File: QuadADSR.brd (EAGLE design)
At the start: 66.6 x 100 mm, 75 parts, among them IC1 74AC32D, IC5 MCP6004D, Q1 20MHz, T1 2N3904, T2 2N3904, T3 2N3904, T4 2N3904, U1 ATMEGA328P, U2 DUAL_OPAMP, U3 7805, U4 4051

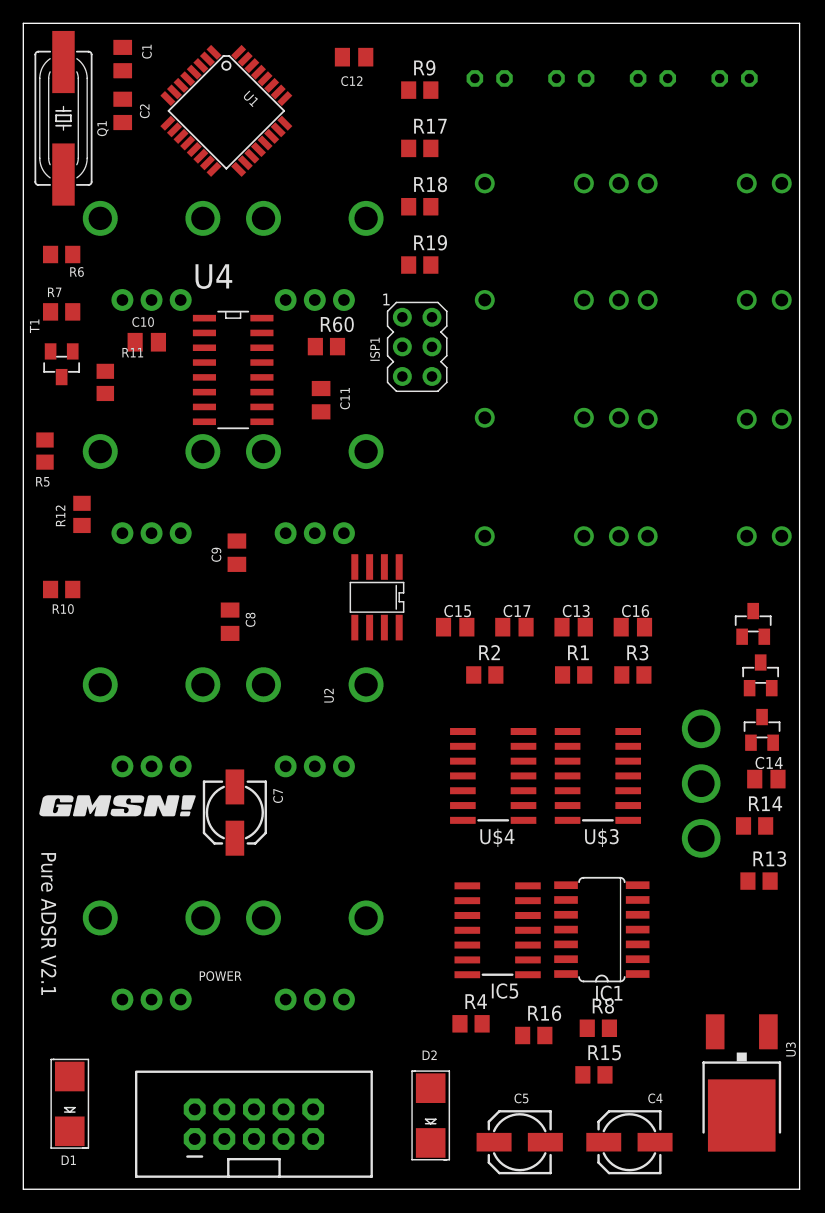
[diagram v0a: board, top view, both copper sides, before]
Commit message: Moved a few thigs round
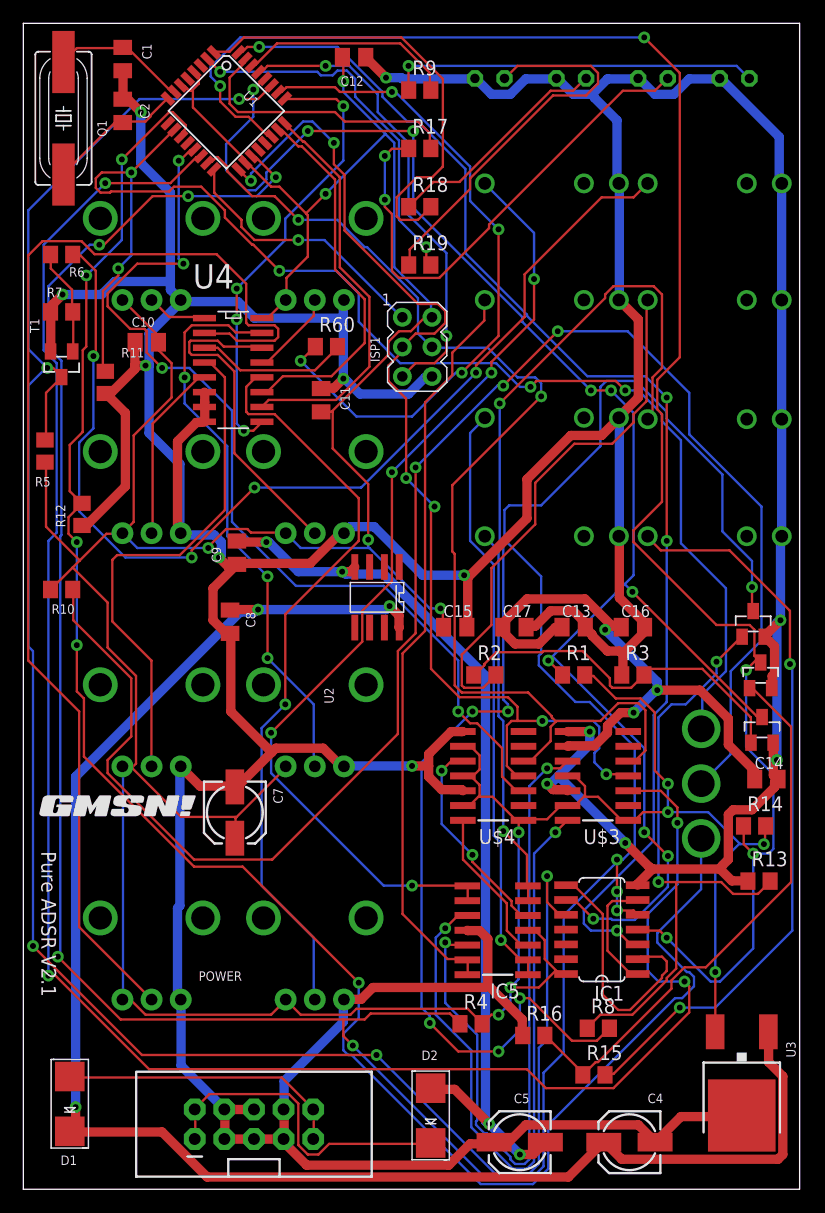
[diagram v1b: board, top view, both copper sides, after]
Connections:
- removed net 3VREF: U$3.11, U$3.13, U$4.11, U$4.13
- removed net N$16: IC1.7
- removed net N$17: IC1.14
- net +5V: now also C15.1, IC1.14, IC5.4, U$3.1, U$3.11, U$3.13, U$4.1, U$4.11, U$4.13, U$4.9
- net 5V: no longer C15.1, IC5.4, U$3.1, U$4.1, U$4.9
- net GND: now also IC1.7
- net TRIG: no longer U1.9
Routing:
- net GND: track 0.00 -> 569.5 mm, vias 0 -> 13
- net +5V: track 0.00 -> 364.9 mm, vias 0 -> 12
- net TRIG3: track 0.00 -> 260.2 mm, vias 0 -> 9
- net TRIG1: track 0.00 -> 178.6 mm, vias 0 -> 5
- net CS1: track 0.00 -> 168.0 mm, vias 0 -> 4
- net T2: track 0.00 -> 161.0 mm, vias 0 -> 5
- net TRIG4: track 0.00 -> 153.9 mm, vias 0 -> 5
- net +12V: track 0.00 -> 144.1 mm, vias 0 -> 3
- net N$12: track 0.00 -> 143.3 mm, vias 0 -> 3
- net TRIG2: track 0.00 -> 139.0 mm, vias 0 -> 10
- net T1: track 0.00 -> 116.8 mm, vias 0 -> 5
- net N$6: track 0.00 -> 110.2 mm, vias 0 -> 6
- net TRIG: track 0.00 -> 107.3 mm, vias 0 -> 4
- net POT_ST: track 0.00 -> 102.7 mm
- net MOSI: track 0.00 -> 96.9 mm, vias 0 -> 2
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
